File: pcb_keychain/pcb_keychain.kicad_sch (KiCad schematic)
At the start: 5 parts, among them U1 13.56MHz

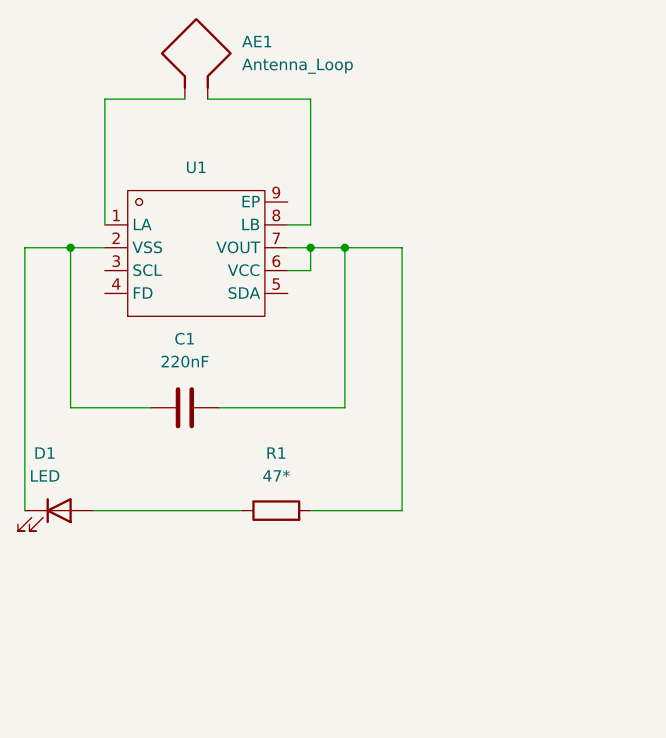
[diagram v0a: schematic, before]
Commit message: updated schematic
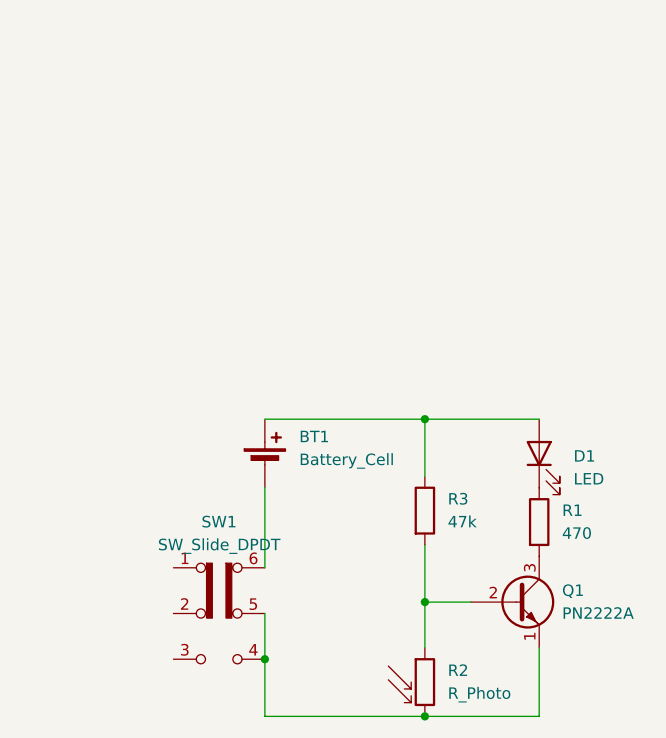
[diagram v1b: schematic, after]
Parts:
- removed AE1: Antenna_Loop, symbol Device:Antenna_Loop
- removed C1: 220nF, symbol Device:C
- removed U1: 13.56MHz, NT3H2111W0FHKH:XQFN-8_L1.6-W1.6-P0.50-BL, symbol JLC_Imports:NT3H2111W0FHKH
- added BT1: Battery_Cell, symbol Device:Battery_Cell
- added Q1: PN2222A, Package_TO_SOT_THT:TO-92_Inline, symbol Transistor_BJT:PN2222A
- added R2: R_Photo, symbol Device:R_Photo
- added R3: 47k, symbol Device:R
- added SW1: SW_Slide_DPDT, symbol Switch:SW_Slide_DPDT
- R1: value 47* -> 470
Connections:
- net at D1.1 (K): now also R1.1
- net at R1.2: now also Q1.3 (C)
- net at D1.2 (A): now also BT1.1 (+), R3.1; no longer R1.1
- new net: Q1.1 (E), R2.2, SW1.4 (A), SW1.5 (B)
- new net: BT1.2 (-), SW1.6 (C)
- new net: Q1.2 (B), R2.1, R3.2
